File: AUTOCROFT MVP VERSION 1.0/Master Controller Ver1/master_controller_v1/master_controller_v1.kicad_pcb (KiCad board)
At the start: 2 copper layers, 120.7 x 133.4 mm, 18 parts, among them J1 DS3231, J2 BME280, J3 ESP8266, J4 HC12, J5 HC06, J6 STM32 Bluepill, J7 Keypad, U1 LM1117-3.3, U2 LM7805_TO220, U3 EEPROM

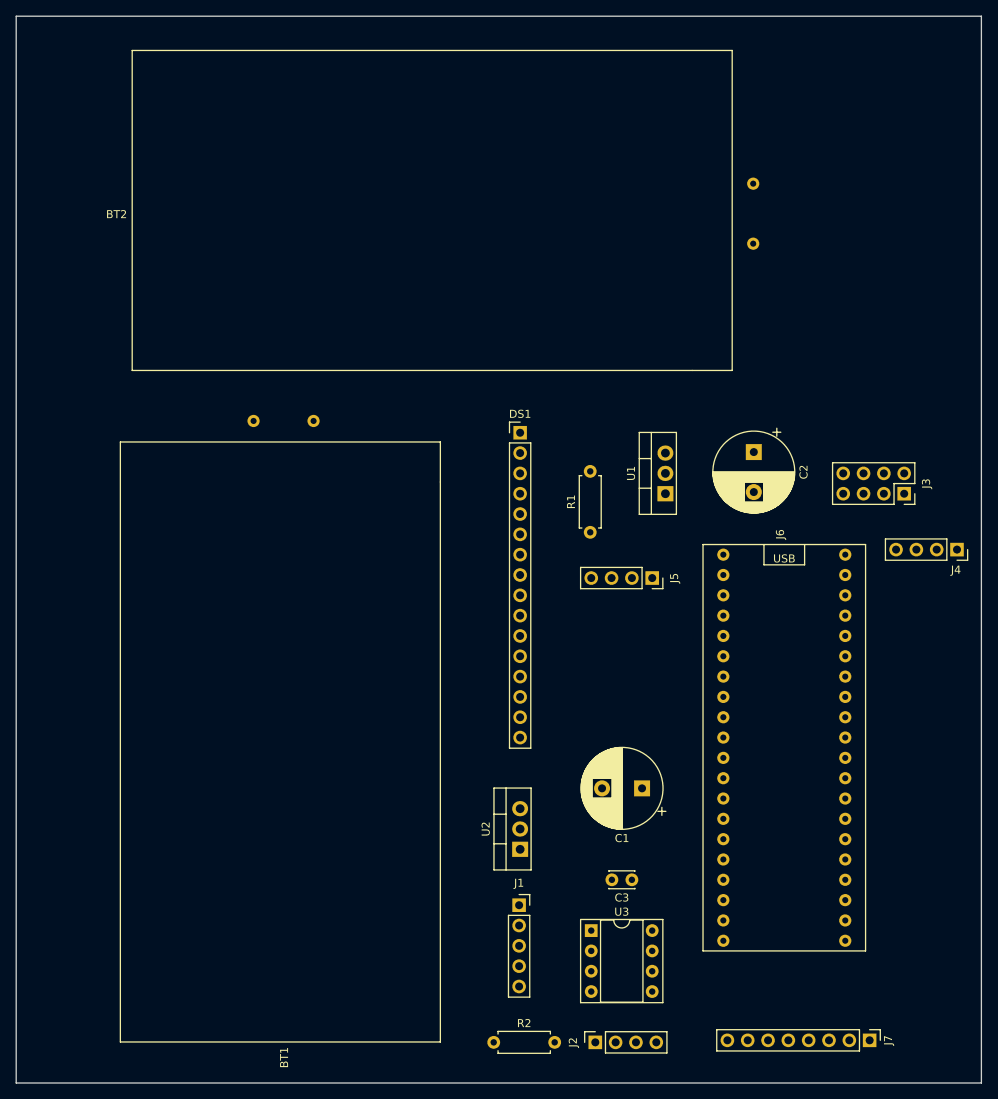
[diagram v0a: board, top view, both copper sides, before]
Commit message: Progress in design
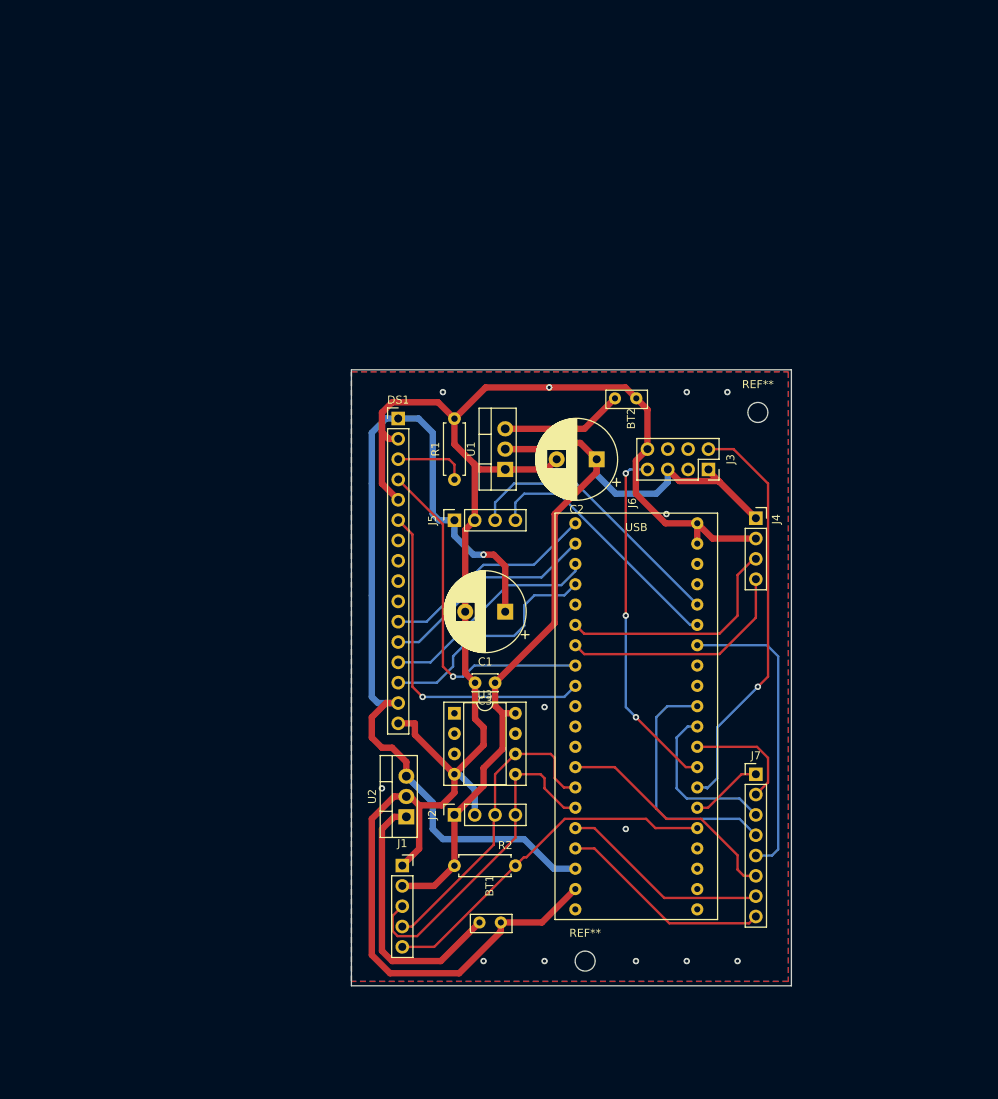
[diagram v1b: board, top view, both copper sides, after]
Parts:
- added REF**: MountingHole_2.5mm, MountingHole:MountingHole_2.5mm, F.Cu at (109.2, 168.9)
- added REF**: MountingHole_2.5mm, MountingHole:MountingHole_2.5mm, F.Cu at (130.8, 100.3)
- moved BT2 68.9 mm to (114.5, 101.1), turned to 90 degrees
- moved J7 36.2 mm to (130.6, 145.6), turned to 0 degrees
- moved J2 33.4 mm to (92.9, 150.6)
- moved U3 32.1 mm to (92.9, 137.9)
- moved BT1 30.1 mm to (97.5, 166.6)
- moved C3 30.0 mm to (98.0, 134.1)
- moved C1 27.9 mm to (99.2, 125.2)
- moved J5 25.8 mm to (92.9, 113.8), turned to 90 degrees
- moved J4 25.5 mm to (130.6, 113.6), turned to 0 degrees
- moved J3 24.7 mm to (124.6, 107.5)
- moved R2 22.2 mm to (100.5, 157.0), turned to 180 degrees
- moved U1 20.3 mm to (99.2, 107.5)
- moved C2 19.7 mm to (110.7, 106.2), turned to 180 degrees
- moved J6 18.9 mm to (115.6, 111.6)
- moved R1 18.2 mm to (92.9, 108.7)
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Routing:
- net GND: track 0.00 -> 232.1 mm, vias 0 -> 13
- net VCC_5V: track 0.00 -> 116.3 mm, vias 0 -> 1
- net VCC_3V3: track 0.00 -> 110.3 mm
- net PA2: track 0.00 -> 51.8 mm, vias 0 -> 1
- net PA3: track 0.00 -> 44.2 mm, vias 0 -> 3
- net PA0: track 0.00 -> 44.0 mm
- net PA11: track 0.00 -> 43.3 mm, vias 0 -> 1
- net PA12: track 0.00 -> 43.0 mm, vias 0 -> 1
- net PB7: track 0.00 -> 42.2 mm
- net PB6: track 0.00 -> 38.9 mm
- net PB1: track 0.00 -> 37.9 mm
- net PB11: track 0.00 -> 34.7 mm
- net Net-(BT1-Pad1): track 0.00 -> 33.6 mm
- net PB10: track 0.00 -> 32.2 mm
- net PA6: track 0.00 -> 30.9 mm
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- added copper zone on B.Cu, net GND
- added copper zone on F.Cu, net GND
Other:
- board size 120.7 x 133.4 mm -> 55 x 77 mm
